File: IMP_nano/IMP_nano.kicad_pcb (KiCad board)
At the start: 2 copper layers, 65.8 x 34.5 mm, 38 parts, among them J1 KF301, J2 Holes, Q1 BC847, Q2 AO3400A, SW1 SW_DPST_x2, SW2 SW_DIP_x04, U1 STM32L051C8T6

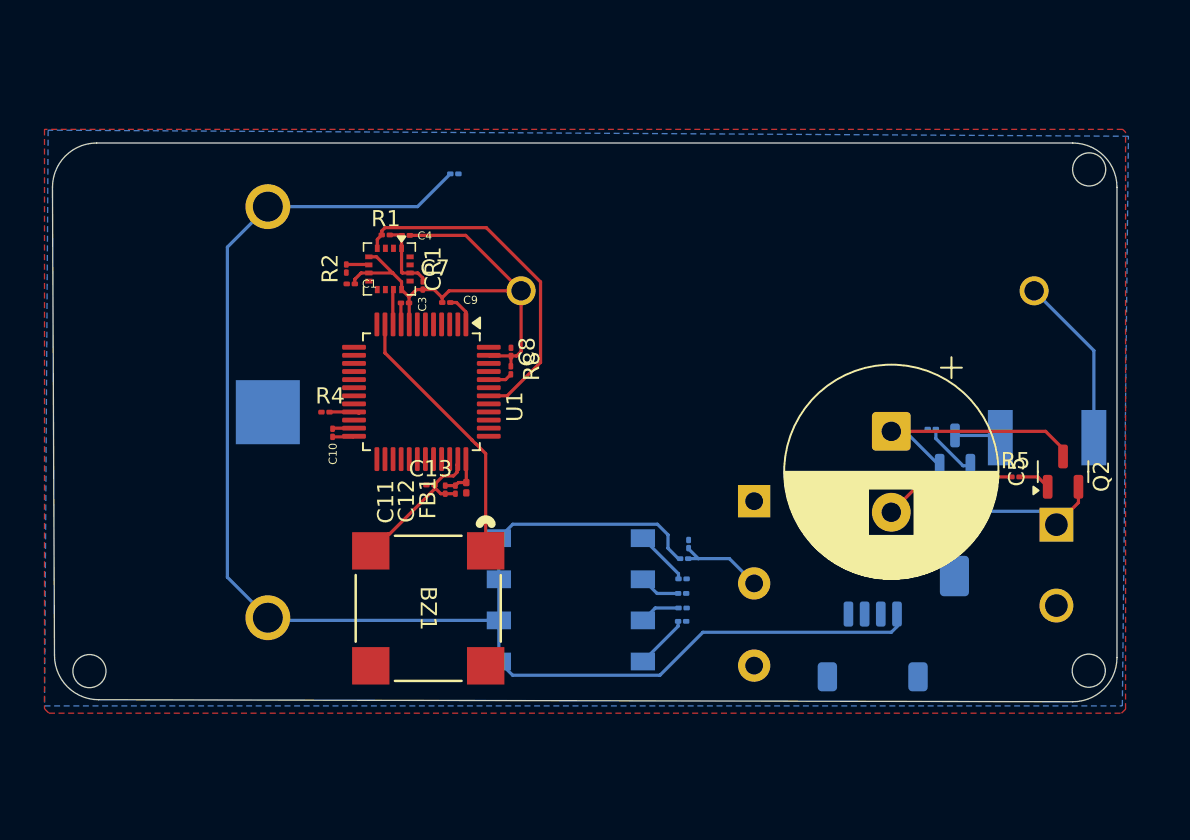
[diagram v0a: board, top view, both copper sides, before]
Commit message: update pcb & schematic
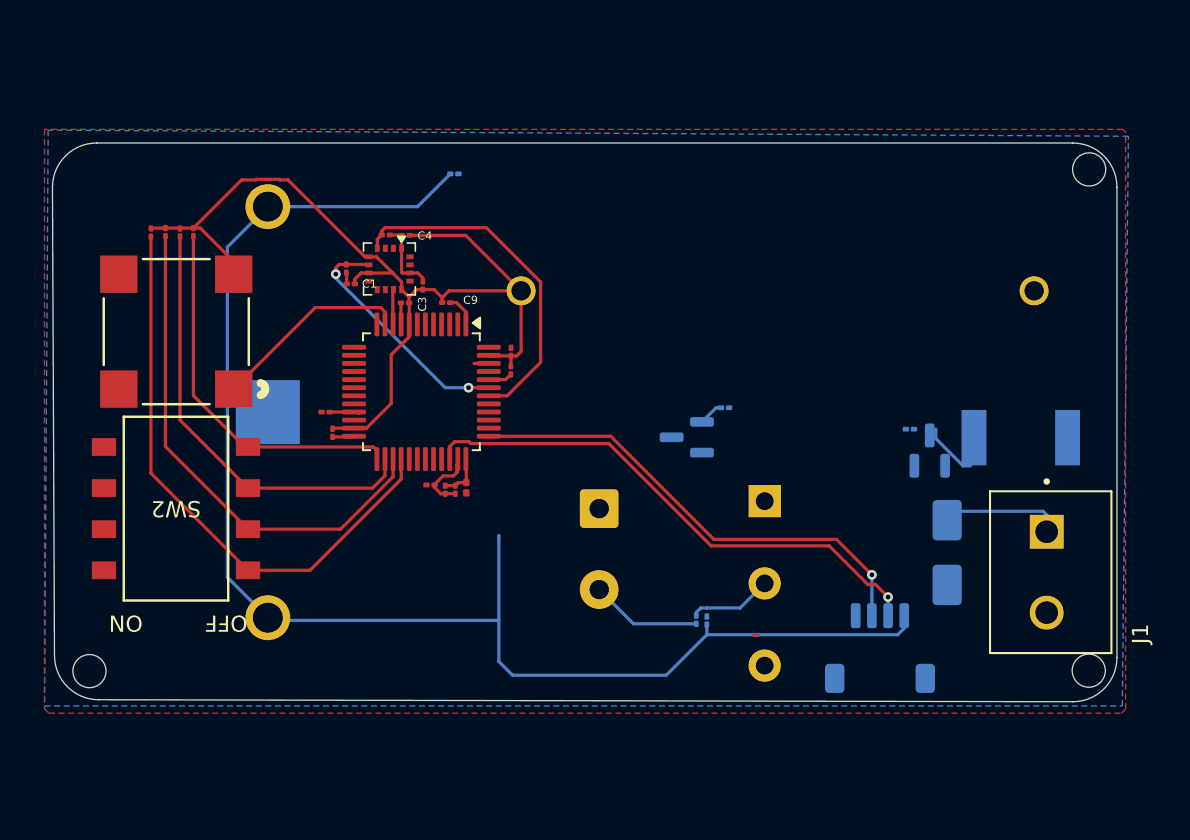
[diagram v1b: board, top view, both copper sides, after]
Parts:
- C5, Q2, R5: moved to B.Cu
- J1, R10, R11, R12, R9, SW2: moved to F.Cu
- moved R12 39.2 mm to (98.8, 79.9), turned to -90 degrees
- moved R11 39.0 mm to (99.7, 79.9), turned to -90 degrees
- moved R10 38.8 mm to (100.6, 79.9), turned to -90 degrees
- moved R9 38.6 mm to (101.4, 79.9), turned to -90 degrees
- moved SW2 25.0 mm to (100.3, 97.0)
- moved Q2 23.3 mm to (131.9, 92.5), turned to 180 degrees
- moved BZ1 23.1 mm to (100.3, 86.0), turned to 180 degrees
- moved C5 18.7 mm to (126.5, 97.0)
- moved R5 18.5 mm to (134.2, 90.7), turned to 180 degrees
- moved C2 4.70 mm to (132.5, 103.8), turned to 90 degrees
- moved R6 4.07 mm to (133.1, 103.9), turned to 90 degrees
- moved R7 1.62 mm to (152.5, 92.6)
- moved Q1 1.56 mm to (146.9, 93.4)
- moved R3 1.35 mm to (145.7, 92.0)
- moved J1 0.74 mm to (154.1, 100.9)
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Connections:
- net +12V renamed /12v
- net BOOT0 renamed /BOOT0
- net BUZ_PWM renamed /BUZ_PWM
- net GPIO_WKP renamed /GPIO_WKP
- net I2C_SCL renamed /I2C_SCL
- net I2C_SDA renamed /I2C_SDA
- net Net-(D1-K) renamed /12v_OUT
- net Net-(Q1-C) renamed /12v_R7
- net Net-(Q1-E) renamed /12v_C5
- R10 pad 2: PB14 -> /M_PB13
- R11 pad 2: PB13 -> /M_PB14
- R12 pad 2: PB12 -> /M_PB15
- R9 pad 2: PB15 -> /M_PB12
- SW2 pad 1: PB12 -> /M_PB15
- SW2 pad 2: PB13 -> /M_PB14
- SW2 pad 3: PB14 -> /M_PB13
- SW2 pad 4: PB15 -> /M_PB12
- U1 pad 25: PB12 -> /M_PB12
- U1 pad 26: PB13 -> /M_PB13
- U1 pad 27: PB14 -> /M_PB14
- U1 pad 28: PB15 -> /M_PB15
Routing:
- net /M_PB15: track 0.00 -> 36.1 mm
- net /SWDIO: track 0.00 -> 33.1 mm, vias 0 -> 1
- net /M_PB14: track 0.00 -> 31.6 mm
- net /SWCLK: track 0.00 -> 29.7 mm, vias 0 -> 1
- net /M_PB13: track 0.00 -> 27.1 mm
- net /M_PB12: track 0.00 -> 23.1 mm
- net GND: track 50.7 -> 72.6 mm
- net /12v_C5: track 15.4 -> 0.00 mm
- net /I2C_SDA: track 1.40 -> 15.0 mm, vias 0 -> 2
- net +3.3V: track 111.0 -> 99.8 mm
- net /12v: track 10.6 -> 0.00 mm
- net /BUZ_PWM: track 16.6 -> 12.3 mm
- net PB12: track 3.43 -> 0.00 mm
- net Net-(Q1-B): track 3.41 -> 0.00 mm
- net PB15: track 3.38 -> 0.00 mm
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
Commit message: fully made pcb & update schematic
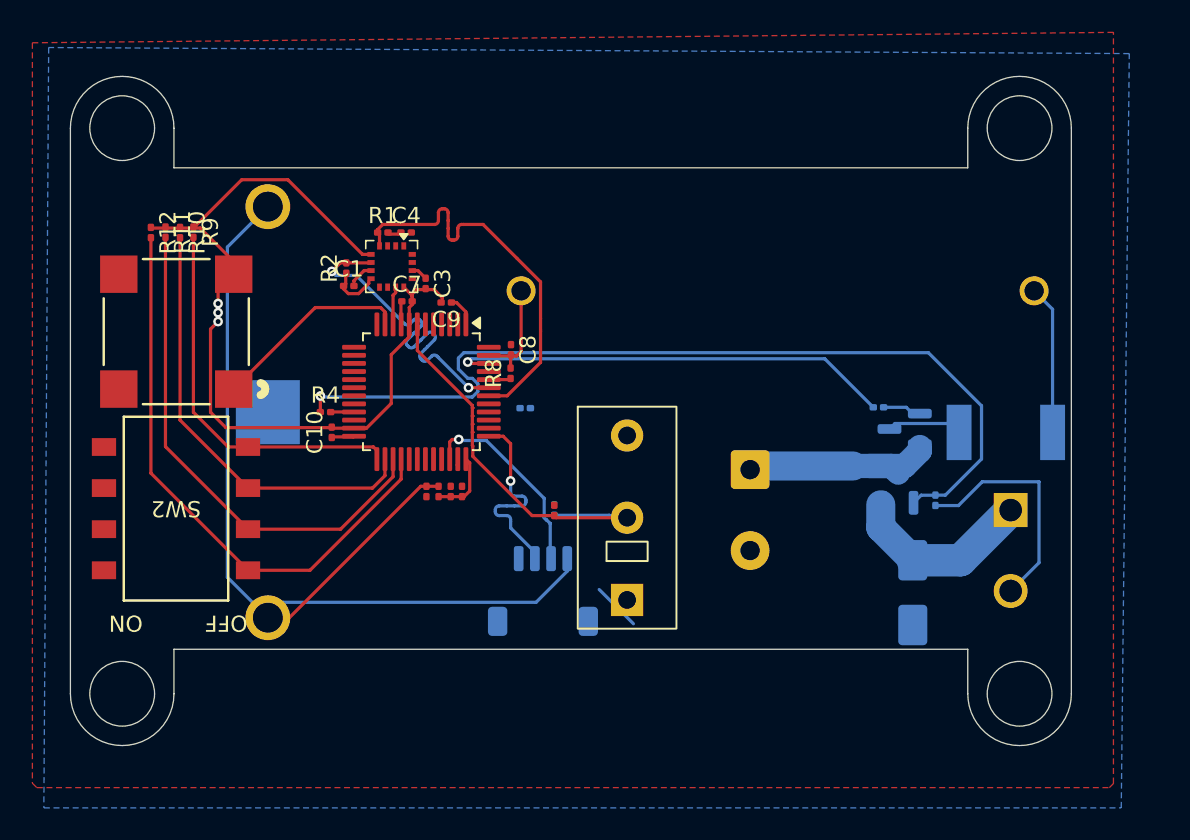
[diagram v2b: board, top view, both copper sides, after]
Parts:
- C1, C10, C11, C12, C13, C2, C3, C4, C6, C7, C8, C9: footprint Capacitor_SMD:C_01005_0402Metric -> Capacitor_SMD:C_0201_0603Metric
- J1: moved to B.Cu
- R1, R10, R11, R12, R2, R3, R4, R5, R8, R9: footprint Resistor_SMD:R_01005_0402Metric -> Resistor_SMD:R_0201_0603Metric
- R6: footprint Resistor_SMD:R_01005_0402Metric -> Resistor_SMD:R_0201_0603Metric; moved to F.Cu
- SW1: moved to F.Cu
- moved J2 21.1 mm to (123.0, 102.0)
- moved C6 15.1 mm to (121.9, 90.8)
- moved R5 14.2 mm to (147.2, 96.4), turned to 90 degrees
- moved Q2 13.4 mm to (144.9, 95.7), turned to 90 degrees
- moved R6 11.6 mm to (123.7, 97.1), turned to -90 degrees
- moved C2 11.1 mm to (123.7, 97.0), turned to -90 degrees
- moved SW1 10.5 mm to (128.2, 102.6), turned to 90 degrees
- moved C5 9.63 mm to (135.8, 94.5)
- moved D1 3.26 mm to (145.8, 102.2)
- moved J1 2.60 mm to (151.9, 99.5)
- moved R3 2.37 mm to (143.7, 90.7)
- moved Q1 2.05 mm to (145.3, 92.0), turned to 180 degrees
- moved FB1 1.73 mm to (116.5, 95.9), turned to -90 degrees
- moved C11 1.04 mm to (118.0, 95.9), turned to 90 degrees
- moved R7 0.98 mm to (151.6, 92.2)
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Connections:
- net Activate renamed /Activate
- net Charge renamed /Charge
- net NRST renamed /NRST
- net Net-(Q1-B) renamed /Q1_1
- net Net-(Q2-G) renamed /Q2_1
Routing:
- net /Q2_1: track 1.54 -> 56.1 mm, vias 0 -> 1
- net +3.3V: track 99.8 -> 71.5 mm
- net /Charge: track 0.91 -> 27.7 mm, vias 0 -> 1
- net /SWDIO: track 33.1 -> 12.4 mm
- net /NRST: track 5.82 -> 23.4 mm
- net /SWCLK: track 29.7 -> 12.4 mm
- net /12v_C5: track 0.00 -> 13.2 mm
- net /12v: track 0.00 -> 9.22 mm
- net GND: track 72.6 -> 80.5 mm, vias 0 -> 3
- net /I2C_SDA: track 15.0 -> 20.8 mm
- net /12v_OUT: track 6.64 -> 11.6 mm
- net /I2C_SCL: track 21.5 -> 24.8 mm
- net /Q1_1: track 0.00 -> 2.40 mm
- net /12v_R7: track 3.41 -> 4.82 mm
- net +3.3VA: track 3.01 -> 4.14 mm
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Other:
- board size 65.8 x 34.5 mm -> 61.9 x 41.4 mm
